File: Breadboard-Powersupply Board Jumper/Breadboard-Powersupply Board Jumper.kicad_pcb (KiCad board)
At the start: 2 copper layers, 17.7 x 9.7 mm, 2 parts, among them J1 Conn_02x02_Odd_Even, J2 Conn_02x02_Odd_Even

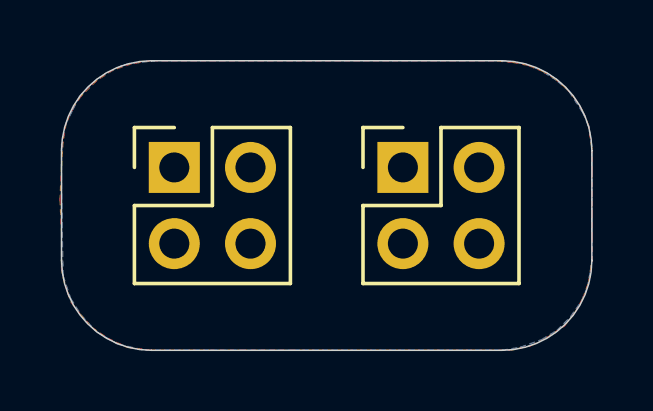
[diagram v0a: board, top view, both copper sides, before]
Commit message: 1-20-23
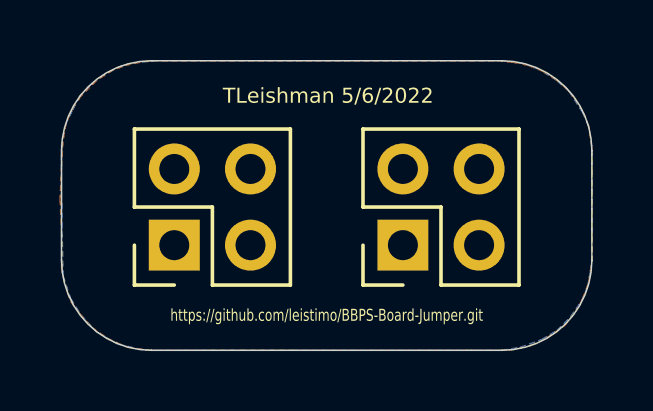
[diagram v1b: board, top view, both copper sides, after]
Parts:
- moved J1 2.59 mm to (139.4, 109.6), turned to 90 degrees
- moved J2 2.59 mm to (147.1, 109.6), turned to 90 degrees
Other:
- board text added: "TLeishman 5/6/2022"
- board text added: "https://github.com/leistimo/BBPS-Board-Jumper.git"
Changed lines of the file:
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@@
   (general
     (thickness 1.6)
-    (drawings 24)
+    (drawings 28)
     (tracks 0)
     (zones 0)
@@
       (outputformat 1)
       (mirror false)
-      (drillshape 1)
+      (drillshape 0)
       (scaleselection 1)
       (outputdirectory ""))
@@
   )
   (module Connector_PinHeader_2.54mm:PinHeader_2x02_P2.54mm_Vertical (layer F.Cu)
-    (at 147.066 107.0356)
+    (at 147.066 109.6264 90)
     (descr "Through hole straight pin header, 2x02, 2.54mm pitch, double rows")
     (tags "Through hole pin header THT 2x02 2.54mm double row")
-    (fp_text reference J2 (at 1.27 -2.33) (layer F.SilkS) hide
-      (effects (font (size 1 1) (thickness 0.15)))
-    )
-    (fp_text value Conn_02x02_Odd_Even (at 1.27 4.87) (layer F.Fab)
-      (effects (font (size 1 1) (thickness 0.15)))
-    )
-    (fp_text user %R (at 1.27 1.27 90) (layer F.Fab)
+    (fp_text reference J2 (at 1.27 -2.33 90) (layer F.SilkS) hide
+      (effects (font (size 1 1) (thickness 0.15)))
+    )
+    (fp_text value Conn_02x02_Odd_Even (at 1.27 4.87 90) (layer F.Fab)
+      (effects (font (size 1 1) (thickness 0.15)))
+    )
+    (fp_text user %R (at 1.27 1.27) (layer F.Fab)
       (effects (font (size 1 1) (thickness 0.15)))
     )
@@
     (fp_line (start 3.81 -1.27) (end 3.81 3.81) (layer F.Fab) (width 0.1))
     (fp_line (start 0 -1.27) (end 3.81 -1.27) (layer F.Fab) (width 0.1))
-    (pad 4 thru_hole oval (at 2.54 2.54) (size 1.7 1.7) (drill 1) (layers *.Cu *.Mask)
-      (net 1 /Power2))
-    (pad 3 thru_hole oval (at 0 2.54) (size 1.7 1.7) (drill 1) (layers *.Cu *.Mask)
-      (net 1 /Power2))
-    (pad 2 thru_hole oval (at 2.54 0) (size 1.7 1.7) (drill 1) (layers *.Cu *.Mask)
-      (net 2 /Power1))
-    (pad 1 thru_hole rect (at 0 0) (size 1.7 1.7) (drill 1) (layers *.Cu *.Mask)
+    (pad 4 thru_hole oval (at 2.54 2.54 90) (size 1.7 1.7) (drill 1) (layers *.Cu *.Mask)
+      (net 1 /Power2))
+    (pad 3 thru_hole oval (at 0 2.54 90) (size 1.7 1.7) (drill 1) (layers *.Cu *.Mask)
+      (net 1 /Power2))
+    (pad 2 thru_hole oval (at 2.54 0 90) (size 1.7 1.7) (drill 1) (layers *.Cu *.Mask)
+      (net 2 /Power1))
+    (pad 1 thru_hole rect (at 0 0 90) (size 1.7 1.7) (drill 1) (layers *.Cu *.Mask)
       (net 2 /Power1))
     (model ${KISYS3DMOD}/Connector_PinHeader_2.54mm.3dshapes/PinHeader_2x02_P2.54mm_Vertical.wrl
@@
   )
   (module Connector_PinHeader_2.54mm:PinHeader_2x02_P2.54mm_Vertical (layer F.Cu)
-    (at 139.446 107.0356)
+    (at 139.446 109.6264 90)
     (descr "Through hole straight pin header, 2x02, 2.54mm pitch, double rows")
     (tags "Through hole pin header THT 2x02 2.54mm double row")
-    (fp_text reference J1 (at 1.27 -2.33) (layer F.SilkS) hide
-      (effects (font (size 1 1) (thickness 0.15)))
-    )
-    (fp_text value Conn_02x02_Odd_Even (at 1.27 4.87) (layer F.Fab)
-      (effects (font (size 1 1) (thickness 0.15)))
-    )
-    (fp_text user %R (at 1.27 1.27 90) (layer F.Fab)
+    (fp_text reference J1 (at 1.27 -2.33 90) (layer F.SilkS) hide
+      (effects (font (size 1 1) (thickness 0.15)))
+    )
+    (fp_text value Conn_02x02_Odd_Even (at 1.27 4.87 90) (layer F.Fab)
+      (effects (font (size 1 1) (thickness 0.15)))
+    )
+    (fp_text user %R (at 1.27 1.27) (layer F.Fab)
       (effects (font (size 1 1) (thickness 0.15)))
     )
@@
     (fp_line (start 3.81 -1.27) (end 3.81 3.81) (layer F.Fab) (width 0.1))
     (fp_line (start 0 -1.27) (end 3.81 -1.27) (layer F.Fab) (width 0.1))
-    (pad 4 thru_hole oval (at 2.54 2.54) (size 1.7 1.7) (drill 1) (layers *.Cu *.Mask)
-      (net 1 /Power2))
-    (pad 3 thru_hole oval (at 0 2.54) (size 1.7 1.7) (drill 1) (layers *.Cu *.Mask)
-      (net 1 /Power2))
-    (pad 2 thru_hole oval (at 2.54 0) (size 1.7 1.7) (drill 1) (layers *.Cu *.Mask)
-      (net 2 /Power1))
-    (pad 1 thru_hole rect (at 0 0) (size 1.7 1.7) (drill 1) (layers *.Cu *.Mask)
+    (pad 4 thru_hole oval (at 2.54 2.54 90) (size 1.7 1.7) (drill 1) (layers *.Cu *.Mask)
+      (net 1 /Power2))
+    (pad 3 thru_hole oval (at 0 2.54 90) (size 1.7 1.7) (drill 1) (layers *.Cu *.Mask)
+      (net 1 /Power2))
+    (pad 2 thru_hole oval (at 2.54 0 90) (size 1.7 1.7) (drill 1) (layers *.Cu *.Mask)
+      (net 2 /Power1))
+    (pad 1 thru_hole rect (at 0 0 90) (size 1.7 1.7) (drill 1) (layers *.Cu *.Mask)
       (net 2 /Power1))
     (model ${KISYS3DMOD}/Connector_PinHeader_2.54mm.3dshapes/PinHeader_2x02_P2.54mm_Vertical.wrl
@@
     )
   )
+  (gr_text "TLeishman 5/6/2022" (at 144.5768 104.648) (layer B.SilkS)
+    (effects (font (size 0.5 0.5) (thickness 0.075)) (justify mirror))
+  )
+  (gr_text "TLeishman 5/6/2022" (at 144.5768 104.648) (layer F.SilkS)
+    (effects (font (size 0.5 0.5) (thickness 0.075)))
+  )
+  (gr_text https://github.com/leistimo/BBPS-Board-Jumper.git (at 144.526 111.9632) (layer B.SilkS)
+    (effects (font (size 0.4 0.3) (thickness 0.0675)) (justify mirror))
+  )
+  (gr_text https://github.com/leistimo/BBPS-Board-Jumper.git (at 144.526 111.9632) (layer F.SilkS)
+    (effects (font (size 0.4 0.3) (thickness 0.0675)))
+  )
   (gr_line (start 153.3652 106.4768) (end 153.3652 110.1344) (layer Edge.Cuts) (width 0.05))
